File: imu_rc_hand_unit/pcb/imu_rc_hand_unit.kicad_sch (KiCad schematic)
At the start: 80 parts, among them J1 USB_C_Receptacle_USB2.0_16P, J2 JST SH1.0, Q1 AO3400A, Q2 AO3400A, Q3 AO3401A, Q4 AO3400A, Q5 AO3401A, Q6 BSS138, Q7 2N2907A, Q8 2N2907A, SW1 SW_SPDT, U1 LSM6DSO, U2 MCP73831, U3 BQ297xy, U4 AP2112K-3.3, U5 ESP32-S3-WROOM-1, U6 CP2102N

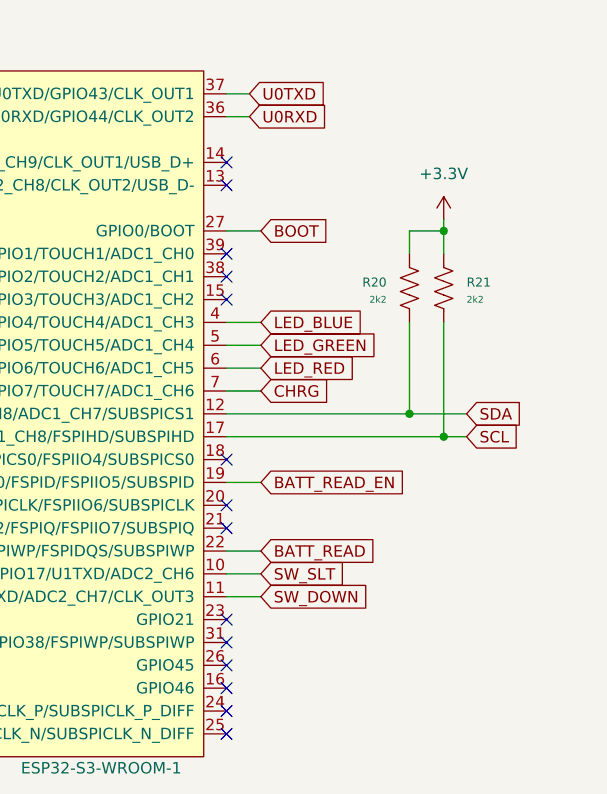
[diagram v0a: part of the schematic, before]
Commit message: commit #12
added cost prevision table #2
minor changes overall
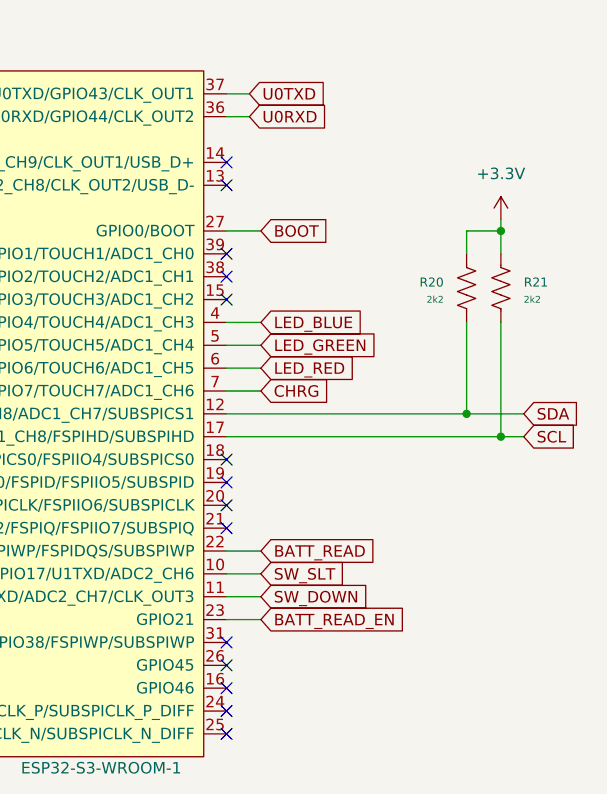
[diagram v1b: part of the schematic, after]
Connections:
- net BATT_READ_EN: now also U5.23 (GPIO21); no longer U5.19 (GPIO11/TOUCH11/ADC2_CH0/FSPID/FSPIIO5/SUBSPID)
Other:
- moved on the sheet: R20, R21
